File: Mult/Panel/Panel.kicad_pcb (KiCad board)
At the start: 2 copper layers, 70.8 x 128.5 mm, 0 parts

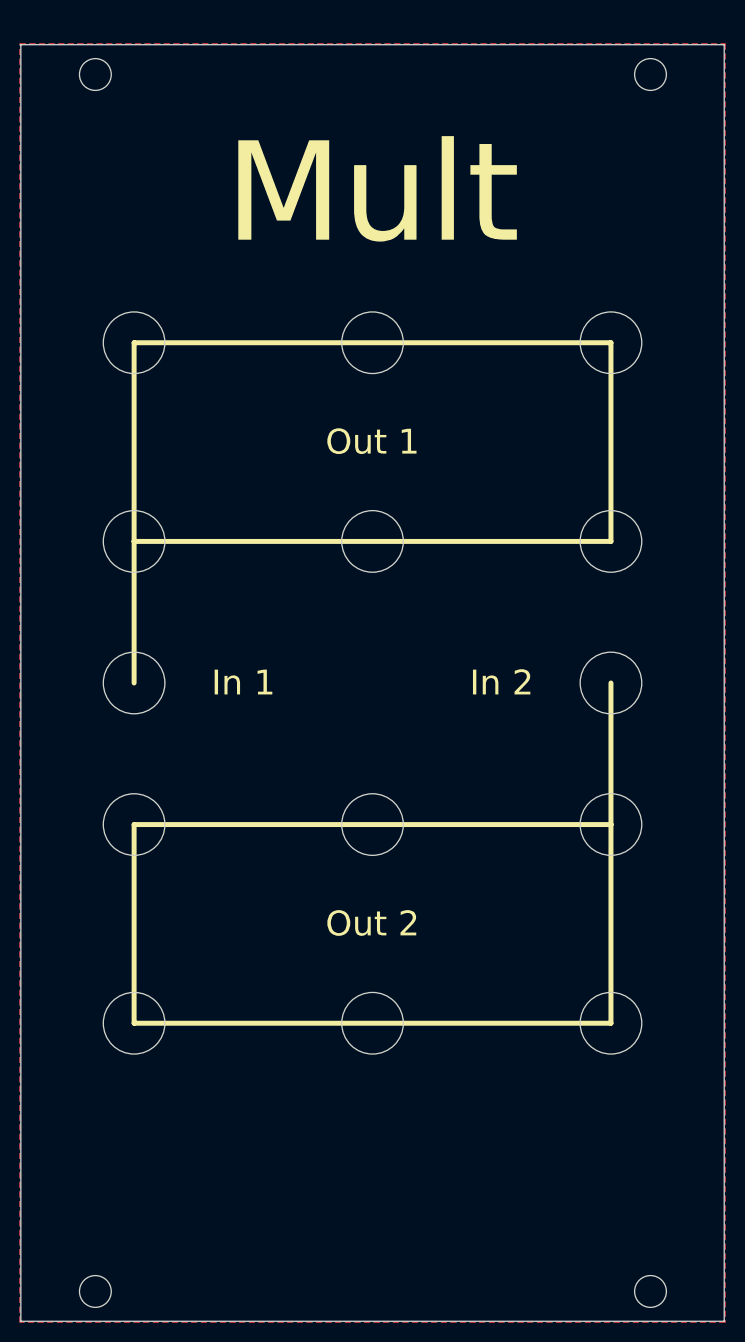
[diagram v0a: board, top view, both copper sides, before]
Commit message: Finish main set of revisions
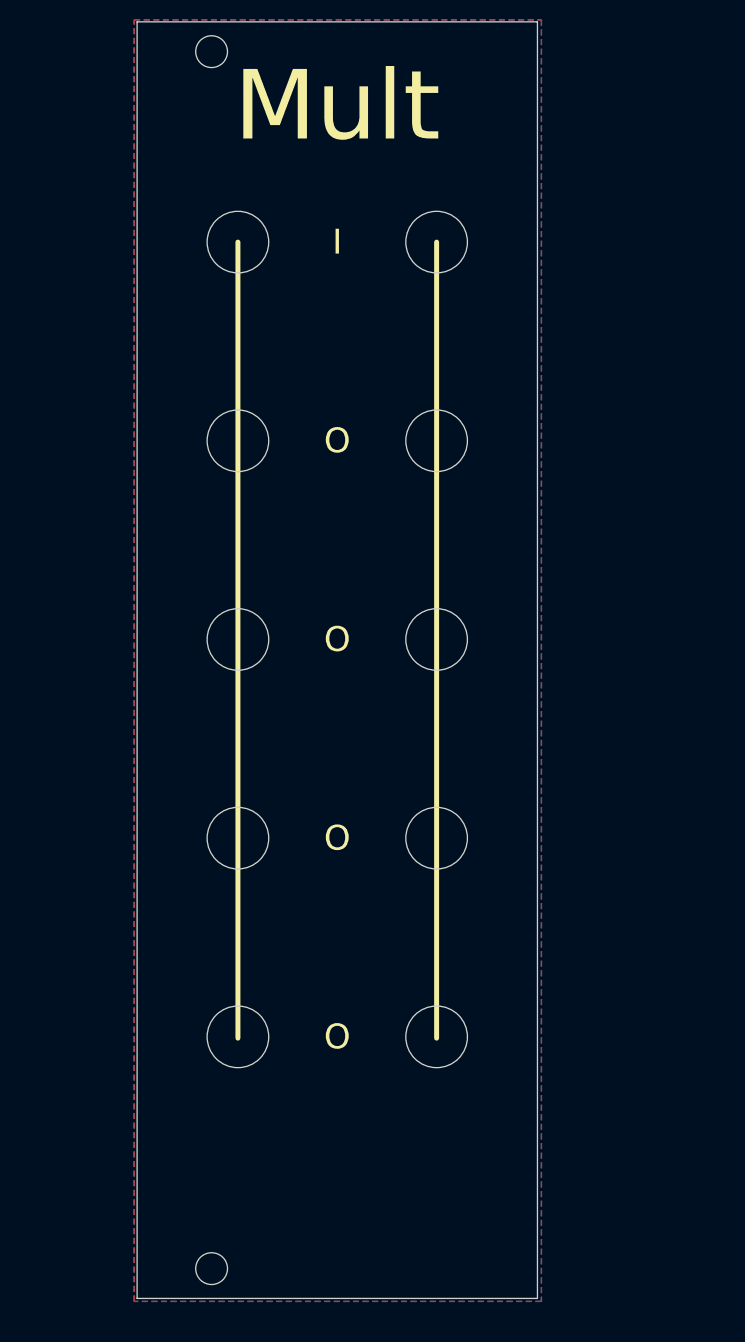
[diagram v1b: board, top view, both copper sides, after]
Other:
- board size 70.8 x 128.5 mm -> 40.3 x 128.5 mm
- board text added: "I"
- board text added: "O"
- board text removed: "In 1"
- board text removed: "In 2"
- board text removed: "Out 1"
- board text removed: "Out 2"
